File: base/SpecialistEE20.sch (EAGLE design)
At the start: 110 parts, among them X1 SCART-F

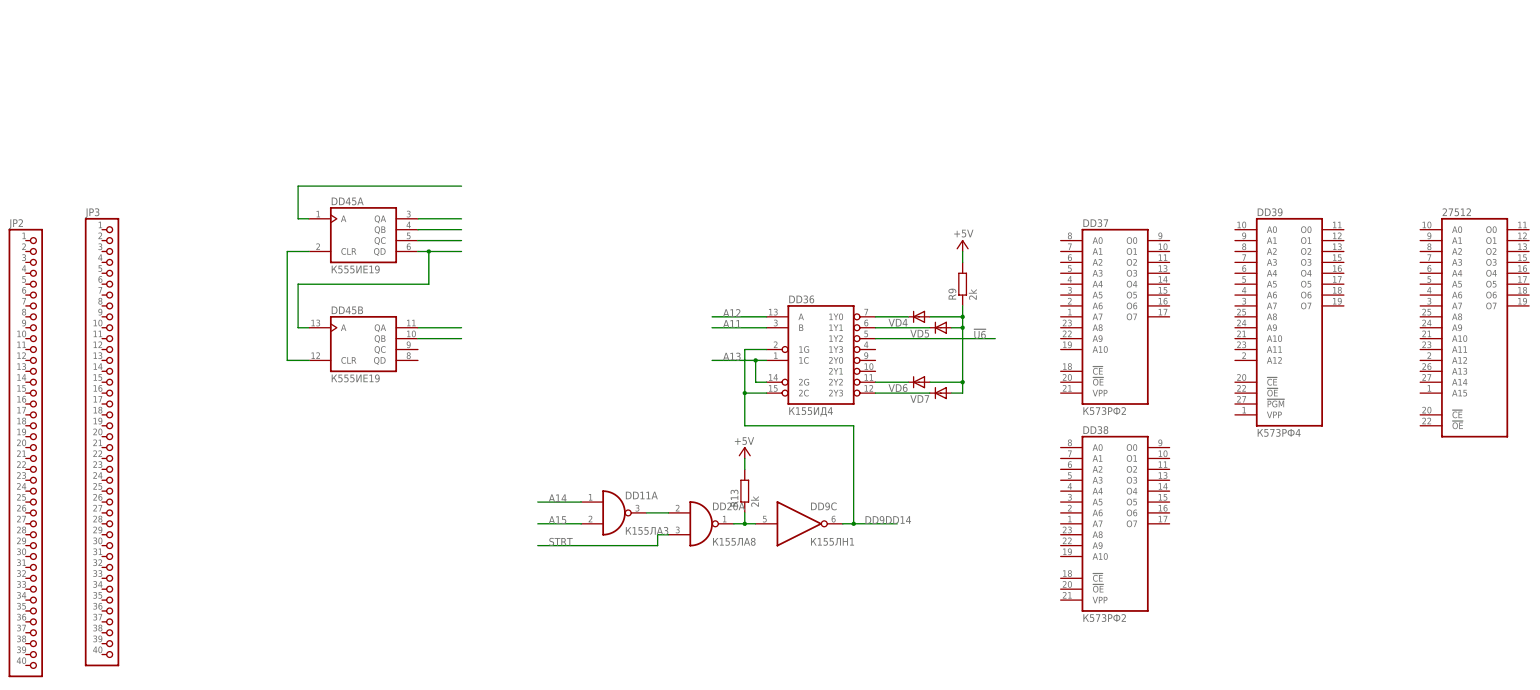
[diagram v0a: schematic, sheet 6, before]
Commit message: .
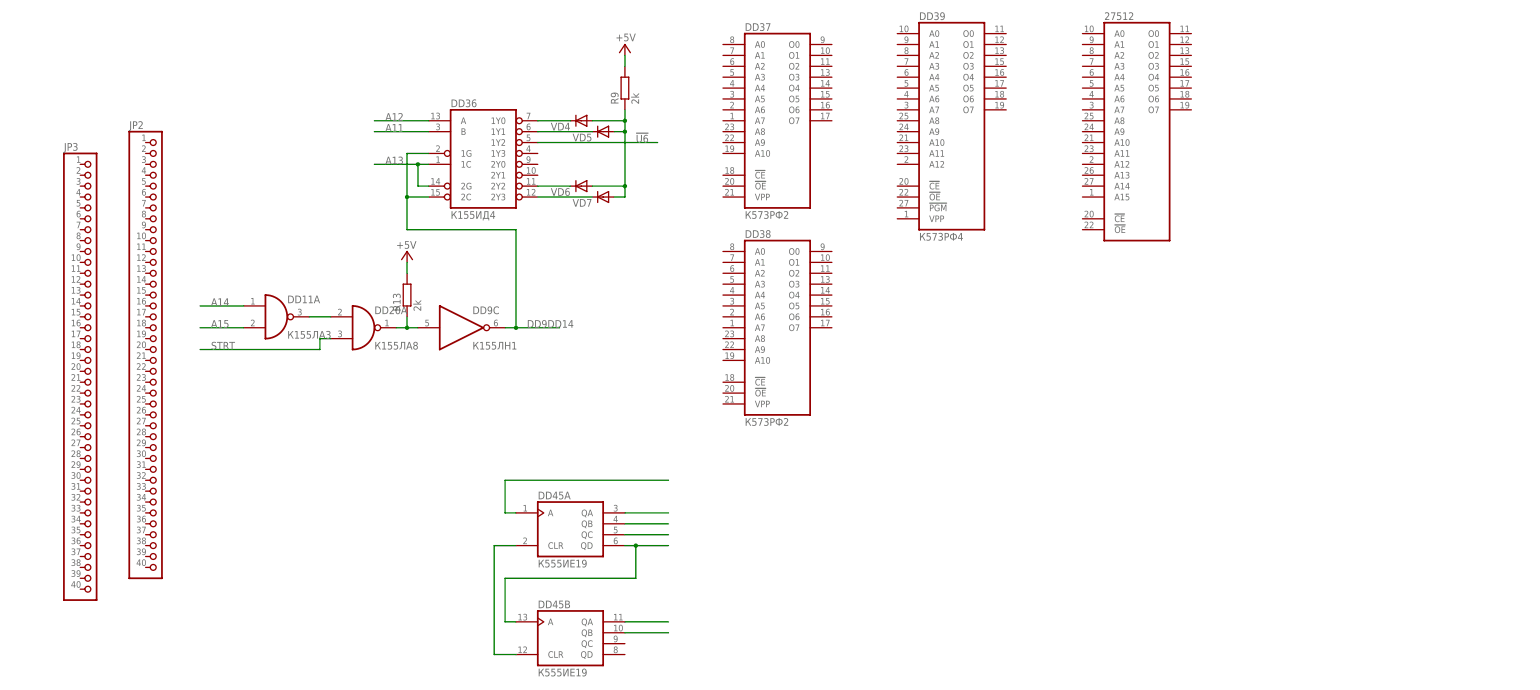
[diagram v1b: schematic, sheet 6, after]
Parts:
- removed DD3011.3: (no value), Разъёмы штырьковые 2.54мм:PINHD-1X20
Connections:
- net !RD: now also DDX12A.5
- net !U6: now also DDX12A.6
- net A0: now also DDX12A.9
- net A1: now also DDX12A.8
- net GND: now also DDX12A.7
- net P1: now also DDX12A.4
- net P10: now also DDX12A.19
- net P11: now also DDX12A.20
- net P12: now also DDX12C.6
- net P13: now also DDX12C.5
- net P14: now also DDX12C.4
- net P15: now also DDX12C.3
- net P16: now also DDX12C.2
- net P17: now also DDX12A.14
- net P18: now also DDX12A.15
- net P19: now also DDX12A.16
- net P2: now also DDX12A.3
- net P20: now also DDX12A.17
- net P21: now also DDX12A.13
- net P22: now also DDX12A.12
- net P23: now also DDX12A.11
- net P24: now also DDX12A.10
- net P3: now also DDX12A.2
- net P4: now also DDX12A.1
- net P5: now also DDX12B.1
- net P6: now also DDX12B.2
- net P7: now also DDX12B.3
- net P8: now also DDX12B.4
- net P9: now also DDX12A.18
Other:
- note added: "PS/2 KB & SD Card"
- note added: "Video"
- moved on the sheet: 27512, DD11A, DD20A, DD36, DD37, DD38, DD39, DD45A, DD45B, DD9C, DDX12B, DDX12C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
